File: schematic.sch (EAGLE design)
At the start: 4 parts, among them U1 ATMEGA328P_TQFP

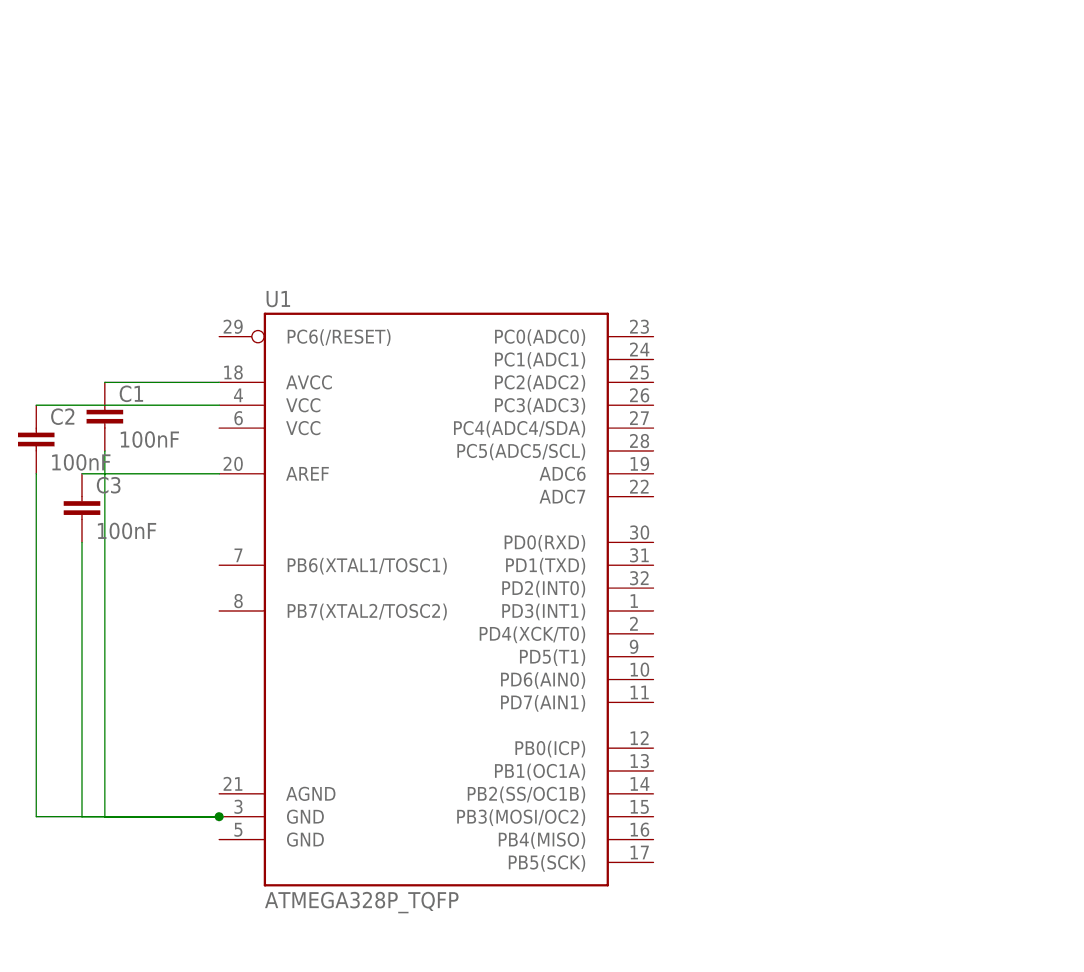
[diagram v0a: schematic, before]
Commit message: Made gitignore
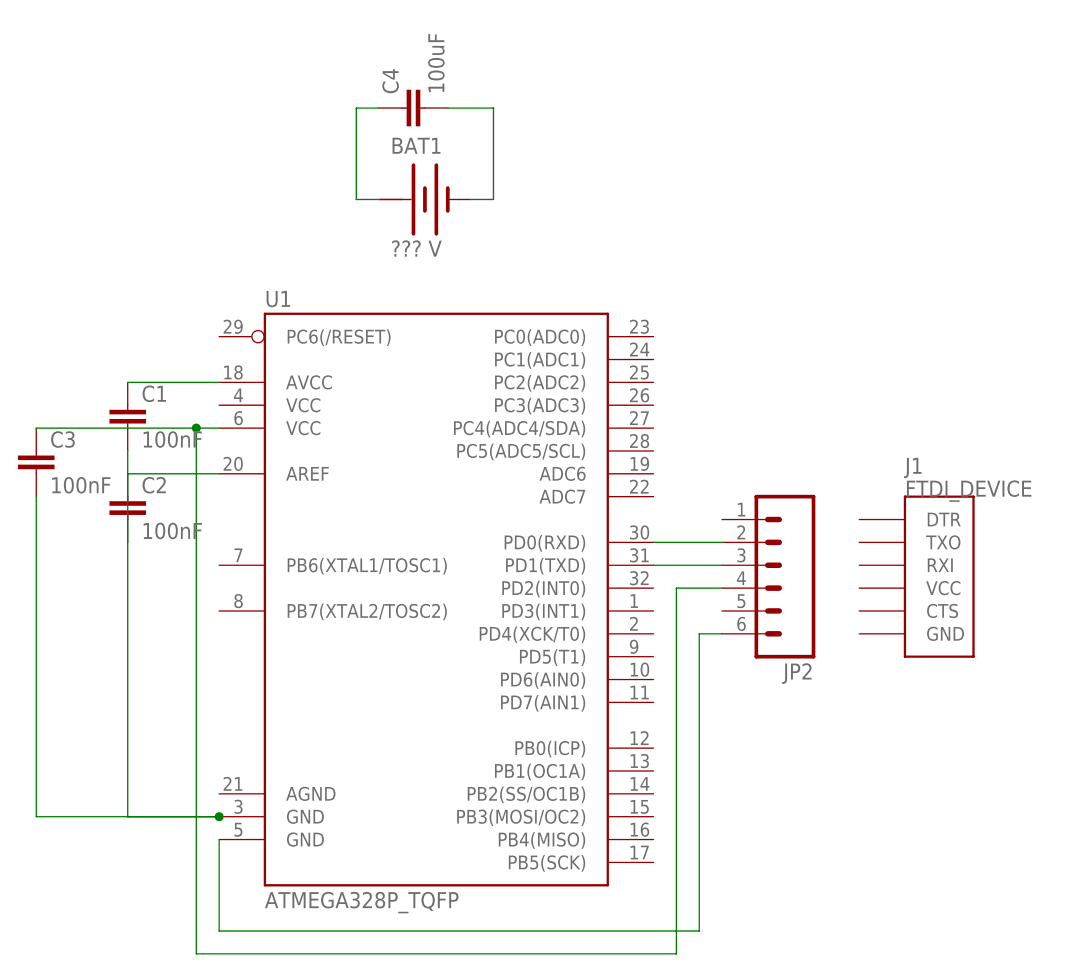
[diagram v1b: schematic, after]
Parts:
- added BAT1: ??? V, special:BATTERY
- added C4: 100uF, rcl:C-EUC2220K
- added J1: FTDI_DEVICE, quad:FTDI_DEVICE
- added JP2: (no value), SparkFun:M06SMD-FEMALE-V2
- C1, C2, C3: device capacitor-wima:C2,5-3 -> rcl:C-EUC0603
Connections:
- new net N$4: JP2.3, U1.PD1(TXD)
- new net N$5: C3.1, JP2.4, U1.VCC@6
- new net N$7: BAT1.-, C4.2
- new net N$8: BAT1.+, C4.1
- new net N$9: JP2.6, U1.GND@5
- net N$2: now also C2.1; no longer C3.1
- net N$3: now also JP2.2, U1.PD0(RXD); no longer C2.1, U1.VCC@4
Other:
- moved on the sheet: C1, C2, C3
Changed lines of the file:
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@@
 <parts>
 <part name="U1" library="quad" deviceset="ATMEGA328P_TQFP" device="" value="ATMEGA328P_TQFP"/>
-<part name="C1" library="capacitor-wima" library_urn="urn:adsk.eagle:library:116" deviceset="C" device="2,5-3" package3d_urn="urn:adsk.eagle:package:5436/1" value="100nF"/>
-<part name="C2" library="capacitor-wima" library_urn="urn:adsk.eagle:library:116" deviceset="C" device="2,5-3" package3d_urn="urn:adsk.eagle:package:5436/1" value="100nF"/>
-<part name="C3" library="capacitor-wima" library_urn="urn:adsk.eagle:library:116" deviceset="C" device="2,5-3" package3d_urn="urn:adsk.eagle:package:5436/1" value="100nF"/>
+<part name="C1" library="rcl" library_urn="urn:adsk.eagle:library:334" deviceset="C-EU" device="C0603" package3d_urn="urn:adsk.eagle:package:23616/2" value="100nF"/>
+<part name="C2" library="rcl" library_urn="urn:adsk.eagle:library:334" deviceset="C-EU" device="C0603" package3d_urn="urn:adsk.eagle:package:23616/2" value="100nF"/>
+<part name="C3" library="rcl" library_urn="urn:adsk.eagle:library:334" deviceset="C-EU" device="C0603" package3d_urn="urn:adsk.eagle:package:23616/2" value="100nF"/>
+<part name="BAT1" library="special" library_urn="urn:adsk.eagle:library:367" deviceset="BATTERY" device="" package3d_urn="urn:adsk.eagle:package:26670/1" value="??? V"/>
+<part name="C4" library="rcl" library_urn="urn:adsk.eagle:library:334" deviceset="C-EU" device="C2220K" package3d_urn="urn:adsk.eagle:package:23687/2" value="100uF"/>
+<part name="J1" library="quad" deviceset="FTDI_DEVICE" device=""/>
+<part name="JP2" library="SparkFun" deviceset="M06" device="SMD-FEMALE-V2"/>
 </parts>
 <sheets>
@@
 <instances>
 <instance part="U1" gate="U$1" x="63.5" y="38.1"/>
-<instance part="C1" gate="G$1" x="25.4" y="60.96"/>
-<instance part="C2" gate="G$1" x="17.78" y="58.42"/>
-<instance part="C3" gate="G$1" x="22.86" y="50.8"/>
+<instance part="C1" gate="G$1" x="27.94" y="60.96"/>
+<instance part="C2" gate="G$1" x="27.94" y="50.8"/>
+<instance part="C3" gate="G$1" x="17.78" y="55.88"/>
+<instance part="BAT1" gate="G$1" x="60.96" y="83.82"/>
+<instance part="C4" gate="G$1" x="58.42" y="93.98" rot="R90"/>
+<instance part="J1" gate="G$1" x="114.3" y="43.18"/>
+<instance part="JP2" gate="G$1" x="99.06" y="43.18" rot="R180"/>
 </instances>
 <busses>
@@
 <pinref part="C1" gate="G$1" pin="1"/>
 <pinref part="U1" gate="U$1" pin="AVCC"/>
-<wire x1="25.4" y1="63.5" x2="38.1" y2="63.5" width="0.1524" layer="91"/>
+<wire x1="27.94" y1="63.5" x2="38.1" y2="63.5" width="0.1524" layer="91"/>
 </segment>
 </net>
 <net name="N$2" class="0">
 <segment>
+<pinref part="C2" gate="G$1" pin="1"/>
+<pinref part="U1" gate="U$1" pin="AREF"/>
+<wire x1="27.94" y1="53.34" x2="38.1" y2="53.34" width="0.1524" layer="91"/>
+</segment>
+</net>
+<net name="N$5" class="0">
+<segment>
 <pinref part="C3" gate="G$1" pin="1"/>
-<pinref part="U1" gate="U$1" pin="AREF"/>
-<wire x1="22.86" y1="53.34" x2="38.1" y2="53.34" width="0.1524" layer="91"/>
+<pinref part="U1" gate="U$1" pin="VCC@6"/>
+<wire x1="17.78" y1="58.42" x2="35.56" y2="58.42" width="0.1524" layer="91"/>
+<pinref part="JP2" gate="G$1" pin="4"/>
+<wire x1="35.56" y1="58.42" x2="38.1" y2="58.42" width="0.1524" layer="91"/>
+<wire x1="93.98" y1="40.64" x2="88.9" y2="40.64" width="0.1524" layer="91"/>
+<wire x1="88.9" y1="40.64" x2="88.9" y2="0" width="0.1524" layer="91"/>
+<wire x1="88.9" y1="0" x2="35.56" y2="0" width="0.1524" layer="91"/>
+<wire x1="35.56" y1="0" x2="35.56" y2="58.42" width="0.1524" layer="91"/>
+<junction x="35.56" y="58.42"/>
+</segment>
+</net>
+<net name="N$6" class="0">
+<segment>
+<pinref part="C2" gate="G$1" pin="2"/>
+<pinref part="U1" gate="U$1" pin="GND@3"/>
+<wire x1="27.94" y1="45.72" x2="27.94" y2="15.24" width="0.1524" layer="91"/>
+<pinref part="C3" gate="G$1" pin="2"/>
+<wire x1="17.78" y1="50.8" x2="17.78" y2="15.24" width="0.1524" layer="91"/>
+<wire x1="17.78" y1="15.24" x2="38.1" y2="15.24" width="0.1524" layer="91"/>
+<junction x="38.1" y="15.24"/>
+<pinref part="C1" gate="G$1" pin="2"/>
+<wire x1="27.94" y1="55.88" x2="27.94" y2="45.72" width="0.1524" layer="91"/>
+<wire x1="27.94" y1="15.24" x2="38.1" y2="15.24" width="0.1524" layer="91"/>
+</segment>
+</net>
+<net name="N$7" class="0">
+<segment>
+<pinref part="BAT1" gate="G$1" pin="-"/>
+<wire x1="66.04" y1="83.82" x2="68.58" y2="83.82" width="0.1524" layer="91"/>
+<wire x1="68.58" y1="83.82" x2="68.58" y2="93.98" width="0.1524" layer="91"/>
+<pinref part="C4" gate="G$1" pin="2"/>
+<wire x1="68.58" y1="93.98" x2="63.5" y2="93.98" width="0.1524" layer="91"/>
+</segment>
+</net>
+<net name="N$8" class="0">
+<segment>
+<pinref part="C4" gate="G$1" pin="1"/>
+<wire x1="55.88" y1="93.98" x2="53.34" y2="93.98" width="0.1524" layer="91"/>
+<wire x1="53.34" y1="93.98" x2="53.34" y2="83.82" width="0.1524" layer="91"/>
+<pinref part="BAT1" gate="G$1" pin="+"/>
+<wire x1="53.34" y1="83.82" x2="55.88" y2="83.82" width="0.1524" layer="91"/>
 </segment>
 </net>
 <net name="N$3" class="0">
 <segment>
-<pinref part="C2" gate="G$1" pin="1"/>
-<pinref part="U1" gate="U$1" pin="VCC@4"/>
-<wire x1="17.78" y1="60.96" x2="38.1" y2="60.96" width="0.1524" layer="91"/>
+<pinref part="JP2" gate="G$1" pin="2"/>
+<pinref part="U1" gate="U$1" pin="PD0(RXD)"/>
+<wire x1="93.98" y1="45.72" x2="86.36" y2="45.72" width="0.1524" layer="91"/>
 </segment>
 </net>
 <net name="N$4" class="0">
 <segment>
-<pinref part="C3" gate="G$1" pin="2"/>
-<pinref part="U1" gate="U$1" pin="GND@3"/>
-<wire x1="22.86" y1="45.72" x2="22.86" y2="15.24" width="0.1524" layer="91"/>
-<wire x1="22.86" y1="15.24" x2="38.1" y2="15.24" width="0.1524" layer="91"/>
-<pinref part="C2" gate="G$1" pin="2"/>
-<wire x1="17.78" y1="53.34" x2="17.78" y2="15.24" width="0.1524" layer="91"/>
-<wire x1="17.78" y1="15.24" x2="38.1" y2="15.24" width="0.1524" layer="91"/>
-<junction x="38.1" y="15.24"/>
-<pinref part="C1" gate="G$1" pin="2"/>
-<wire x1="25.4" y1="55.88" x2="25.4" y2="15.24" width="0.1524" layer="91"/>
-<wire x1="25.4" y1="15.24" x2="38.1" y2="15.24" width="0.1524" layer="91"/>
+<pinref part="JP2" gate="G$1" pin="3"/>
+<pinref part="U1" gate="U$1" pin="PD1(TXD)"/>
+<wire x1="93.98" y1="43.18" x2="86.36" y2="43.18" width="0.1524" layer="91"/>
 </segment>
 </net>
+<net name="N$9" class="0">
+<segment>
+<pinref part="JP2" gate="G$1" pin="6"/>
+<wire x1="93.98" y1="35.56" x2="91.44" y2="35.56" width="0.1524" layer="91"/>
+<wire x1="91.44" y1="35.56" x2="91.44" y2="2.54" width="0.1524" layer="91"/>
+<wire x1="91.44" y1="2.54" x2="38.1" y2="2.54" width="0.1524" layer="91"/>
+<pinref part="U1" gate="U$1" pin="GND@5"/>
+<wire x1="38.1" y1="2.54" x2="38.1" y2="12.7" width="0.1524" layer="91"/>
+</segment>
+</net>
